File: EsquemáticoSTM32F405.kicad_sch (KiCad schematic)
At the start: 31 parts, among them CN4 0430450400, P1 PZ254R-12-8P, SW1 EVQPLMA15, SW2 EVQPLMA15, U1 STM32F405RGT6, X1 32.768kHz 7pF SMD, X2 8Mhz 10pF

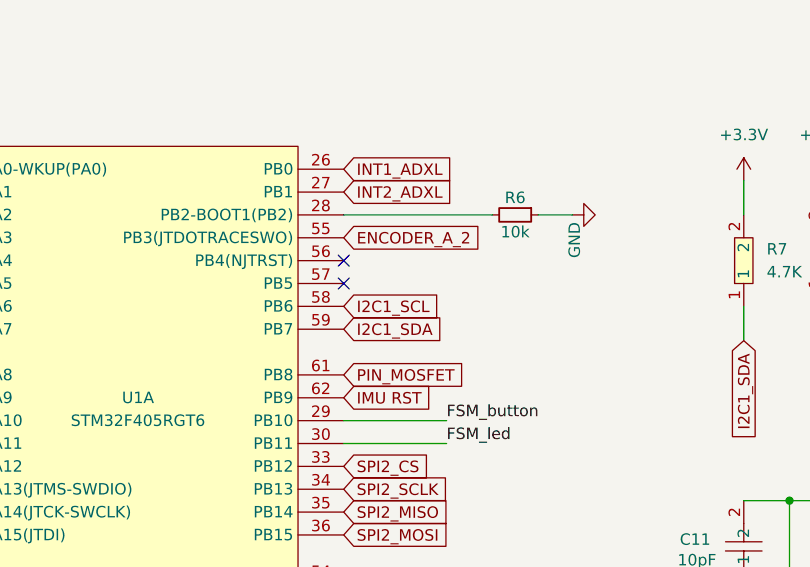
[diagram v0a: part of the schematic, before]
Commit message: 08/08
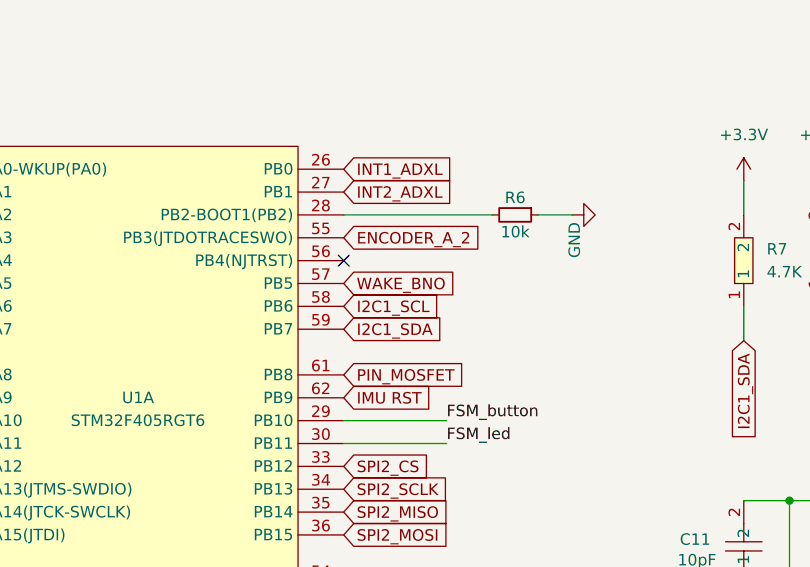
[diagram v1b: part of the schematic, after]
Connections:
- net WAKE_BNO: now reaches U1.57 (PB5)
- no-connect marks 10 -> 9
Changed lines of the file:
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@@
 	)
 	(no_connect
-		(at 302.26 146.05)
-	)
-	(no_connect
 		(at 302.26 179.07)
 	)
@@
 			)
 		)
+	)
+	(global_label "WAKE_BNO"
+		(shape input)
+		(at 302.26 146.05 0)
+		(fields_autoplaced yes)
+		(effects
+			(font
+				(size 1.27 1.27)
+			)
+			(justify left)
+		)
+		(property "Intersheetrefs" "${INTERSHEET_REFS}"
+			(at 315.1028 146.05 0)
+			(hide yes)
+			(show_name no)
+			(do_not_autoplace no)
+			(effects
+				(font
+					(size 1.27 1.27)
+				)
+				(justify left)
+			)
+		)
